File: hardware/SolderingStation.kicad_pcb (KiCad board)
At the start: 2 copper layers, 100 x 100 mm, 96 parts, among them J1 AC Screw Terminal, J10 Power, J11 Logic, J12 SWD, J13 Relay Contact, J14 Relay Coil, J2 Iron Encoder, J3 Hot Air Encoder, J4 OLED, J5 High Voltage, J6 UART, J7 STM BOOT, J8 +5V, J9 Logic, Q1 IRLZ44N, Q2 S8050, Q3 S8050, Q5 S8050, Q6 AO3400A, Q7 BTA16-600B, SW1 SW_SPST, SW2 SW_SPST, SW3 SW_SPST, U1 MOC3063M, U2 AMS1117-3.3, U4 AMS1117-3.3, U5 STM32F103C8Tx, U6 MCP6002-xSN, U7 ADS1115, Y2 Crystal_GND24_Small

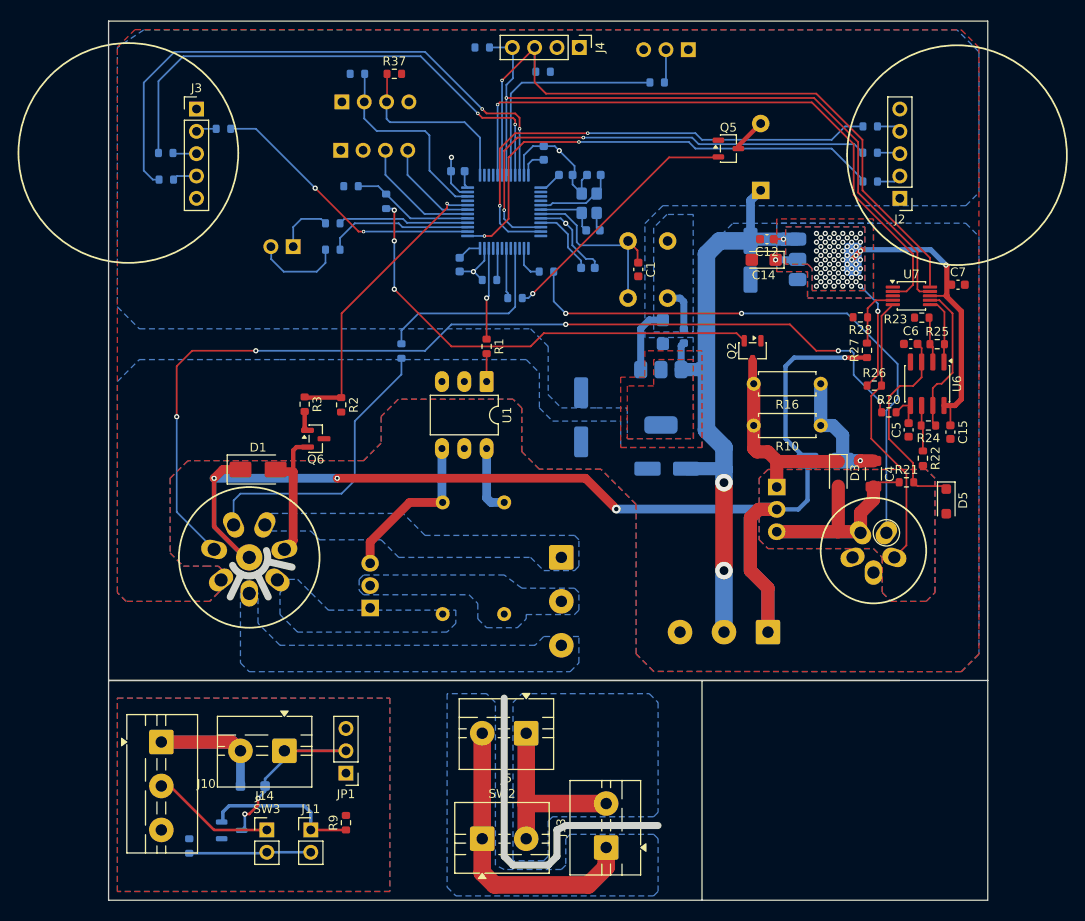
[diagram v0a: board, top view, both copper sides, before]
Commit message: last
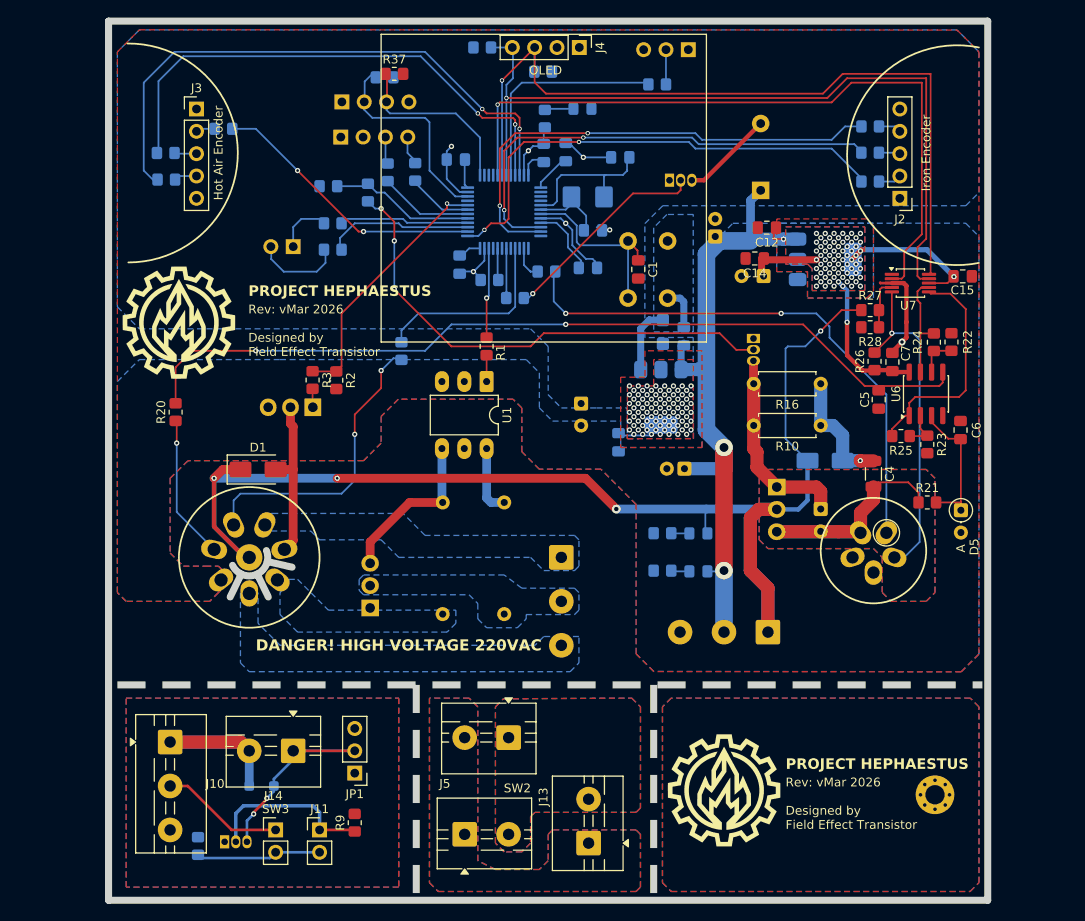
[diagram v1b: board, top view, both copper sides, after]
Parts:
- removed Q6: AO3400A, Package_TO_SOT_SMD:SOT-23
- removed Y2: Crystal_GND24_Small, Crystal:Crystal_SMD_3225-4Pin_3.2x2.5mm
- added C21: 100uF, Capacitor_THT:CP_Radial_D6.3mm_P2.50mm, B.Cu at (119.5, 74.0)
- added C8: 0.1u, Capacitor_SMD:C_0805_2012Metric_Pad1.18x1.45mm_HandSolder, B.Cu at (103.0, 92.9)
- added D6: LED, LED_SMD:LED_0805_2012Metric_Pad1.15x1.40mm_HandSolder, B.Cu at (98.9, 55.0)
- added D7: LED, LED_SMD:LED_0805_2012Metric_Pad1.15x1.40mm_HandSolder, B.Cu at (112.1, 107.6)
- added D8: LED, LED_SMD:LED_0805_2012Metric_Pad1.15x1.40mm_HandSolder, B.Cu at (112.1, 103.3)
- added G***: LOGO, SolderingStationLib:logo, F.Cu at (53.0, 79.3)
- added G***: LOGO, SolderingStationLib:logo, F.Cu at (115.0, 132.5)
- added G***: LOGO, SolderingStationLib:QRcode, B.Cu at (115.0, 132.5)
- added Q4: IRLZ44N, Package_TO_SOT_THT:TO-220-3_Vertical, B.Cu at (68.2, 88.9)
- added R38: 1k, Resistor_SMD:R_0805_2012Metric_Pad1.20x1.40mm_HandSolder, B.Cu at (94.6, 56.1)
- added R39: 2.2k, Resistor_SMD:R_0805_2012Metric_Pad1.20x1.40mm_HandSolder, B.Cu at (108.0, 107.5)
- added R40: 10k, Resistor_SMD:R_0805_2012Metric_Pad1.20x1.40mm_HandSolder, B.Cu at (108.0, 103.2)
- added R41: 1k, Resistor_SMD:R_0805_2012Metric_Pad1.20x1.40mm_HandSolder, B.Cu at (76.8, 62.2)
- added R42: 1k, Resistor_SMD:R_0805_2012Metric_Pad1.20x1.40mm_HandSolder, B.Cu at (79.9, 62.1)
- added REF**: MountingHole_2.2mm_M2_Pad_Via, MountingHole:MountingHole_2.2mm_M2_Pad_Via, F.Cu at (139.0, 133.0)
- added Y1: X50328MSB2GI, Crystal:Crystal_SMD_5032-2Pin_5.0x3.2mm, B.Cu at (99.5, 65.0)
- C1, C10, C12, C15, C16, C17, C18, C19, C2, C20, C6, C7, C9: footprint Capacitor_SMD:C_0603_1608Metric -> Capacitor_SMD:C_0805_2012Metric_Pad1.18x1.45mm_HandSolder
- C11: footprint Capacitor_SMD:CP_Elec_6.3x5.4 -> Capacitor_THT:CP_Radial_D6.3mm_P2.50mm
- C13, C3: footprint Capacitor_SMD:CP_Elec_5x5.4 -> Capacitor_THT:CP_Radial_D5.0mm_P2.00mm
- C14: value 22uF -> 0.1u; footprint Capacitor_Tantalum_SMD:CP_EIA-3216-18_Kemet-A -> Capacitor_SMD:C_0805_2012Metric_Pad1.18x1.45mm_HandSolder
- C4: value 10uF 50V -> 10uF
- C5: value 1u -> 1uF; footprint Capacitor_SMD:C_0603_1608Metric -> Capacitor_SMD:C_0805_2012Metric_Pad1.18x1.45mm_HandSolder
- D3: footprint Diode_SMD:D_SOD-123F -> Diode_THT:D_DO-35_SOD27_P2.54mm_Vertical_AnodeUp; moved to B.Cu
- D5: footprint Diode_SMD:D_SOD-123F -> Diode_THT:D_DO-35_SOD27_P2.54mm_Vertical_AnodeUp
- Q2, Q5: value S8050 -> 2N2222; footprint Package_TO_SOT_SMD:SOT-23-3 -> Package_TO_SOT_THT:TO-92_Inline; moved to B.Cu
- Q3: value S8050 -> 2N2222; footprint Package_TO_SOT_SMD:SOT-23-3 -> Package_TO_SOT_THT:TO-92_Inline
- R1, R11, R12, R13, R14, R15, R17, R18, R19, R2, R20, R21, R22, R23, R24, R25, R26, R27, R28, R29, R3, R30, R31, R32, R33, R34, R35, R36, R37, R6, R7, R8, R9: footprint Resistor_SMD:R_0603_1608Metric -> Resistor_SMD:R_0805_2012Metric_Pad1.20x1.40mm_HandSolder
- moved R20 81.1 mm to (52.6, 89.5), turned to 90 degrees
- moved C15 17.8 mm to (142.2, 74.0), turned to 0 degrees
- moved R23 14.4 mm to (138.1, 93.2), turned to -90 degrees
- moved R22 13.6 mm to (140.9, 81.5), turned to 90 degrees
- moved C7 11.5 mm to (134.2, 83.8), turned to 90 degrees
- moved C6 11.3 mm to (141.9, 91.5), turned to 90 degrees
- moved R25 11.2 mm to (135.1, 92.2), turned to 180 degrees
- moved R24 9.50 mm to (138.9, 81.5), turned to -90 degrees
- moved Q5 7.61 mm to (108.8, 63.1)
- moved C5 4.85 mm to (132.6, 88.0)
- moved C13 4.84 mm to (114.0, 69.5), turned to 90 degrees
- moved R27 4.59 mm to (131.6, 77.9), turned to 0 degrees
- moved D3 4.47 mm to (126.0, 100.5)
- moved C10 3.61 mm to (103.2, 60.5)
- moved R21 3.30 mm to (138.1, 99.8)
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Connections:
- U5 pad 30: /UART_TX -> Net-(U5-PA9)
- U5 pad 31: /UART_RX -> Net-(U5-PA10)
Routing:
- net /TC_AIR: track 111.0 -> 16.4 mm, vias 5 -> 1
- net Net-(U6B-+): track 4.24 -> 97.6 mm, vias 0 -> 2
- net /Safety Relay/INPUT: track 33.6 -> 0.00 mm
- net /Safety Relay/OUTPUT: track 21.1 -> 0.00 mm
- net Net-(U7-AIN2): track 7.74 -> 26.1 mm
- net Net-(U5-PA9): track 0.00 -> 11.2 mm
- net /UART_TX: track 14.0 -> 3.37 mm
- net GNDREF: track 51.7 -> 61.6 mm, vias 4 -> 7
- net /OLED_SDA: track 80.6 -> 90.5 mm
- net /Main Unit/SMPL_RDY: track 72.0 -> 81.7 mm
- net /OLED_SCL: track 82.8 -> 92.2 mm
- net /3V3_STM: track 18.7 -> 27.7 mm, vias 0 -> 90
- net /Logic Power Supply/3V3_ANALOG: track 50.2 -> 41.7 mm, vias 75 -> 74
- net /UART_RX: track 11.3 -> 3.33 mm
- net Net-(D5-K): track 23.6 -> 15.8 mm
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- added copper zone on B.Cu, net (none)
- added copper zone on F.Cu, net (none)
- added copper zone on F.Cu, net /Safety Relay/INPUT
- added copper zone on F.Cu, net /Safety Relay/OUTPUT
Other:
- outline, holes or cut-outs redrawn
- board text added: "DANGER! HIGH VOLTAGE 220VAC"
- board text added: "Hot Air Encoder"
- board text added: "Iron Encoder"
- board text added: "Logic"
- board text added: "OLED"
- board text added: "PROJECT HEPHAESTUS"
- board text added: "Rev: vMar 2026 Designed by Field Effect Transistor"
- board text added: "STM BOOT"
- board text added: "SWD"
- board text added: "UART"
